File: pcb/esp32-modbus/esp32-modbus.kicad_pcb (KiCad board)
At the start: 2 copper layers, 77.5 x 77.9 mm, 54 parts, among them J1 Conn_01x01_Male, J10 Conn_01x01_Male, J12 Conn_01x01_Male, J13 Conn_01x01_Male, J2 Conn_01x05_Male, J22 Conn_01x01_Male, J23 Conn_01x01_Male, J24 Conn_01x01_Male, J25 Conn_01x01_Male, J26 Conn_01x01_Male, J27_VCC1 Conn_01x01_Male, J28_RO1 Conn_01x01_Male, J29_DI1 Conn_01x01_Male, J3 Conn_01x01_Male, J30_RE/DE1 Conn_01x01_Male, J31_GND1 Conn_01x01_Male, J4 Conn_01x01_Male, J5 Conn_01x01_Male, J6 Screw_Terminal_01x02, J7 Conn_01x09_Male, J8 Conn_01x09_Male, J9 Conn_01x01_Male, Q1 BC817, Q2 BC817, U1 ESP32-WROOM-32U

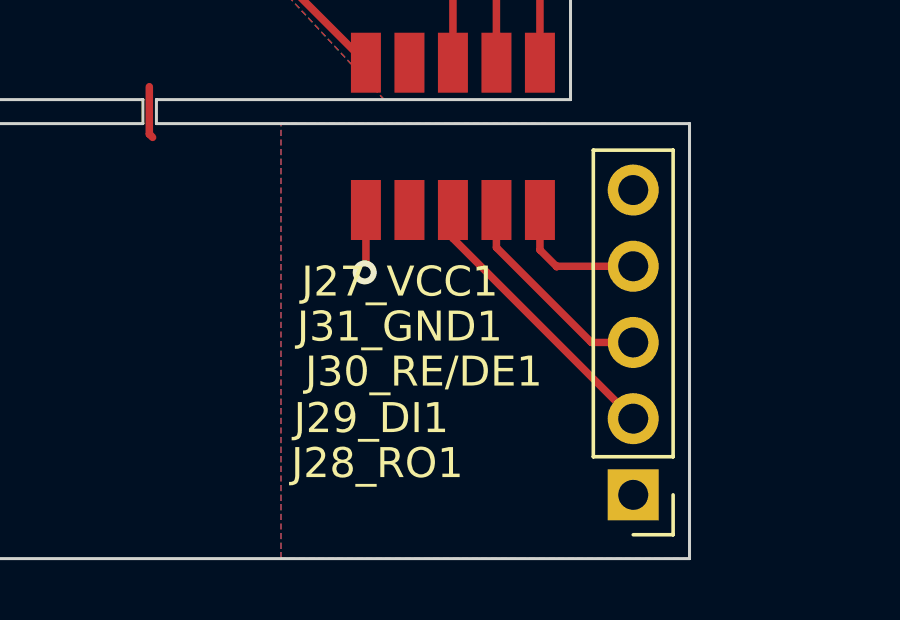
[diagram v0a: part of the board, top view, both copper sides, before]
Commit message: update
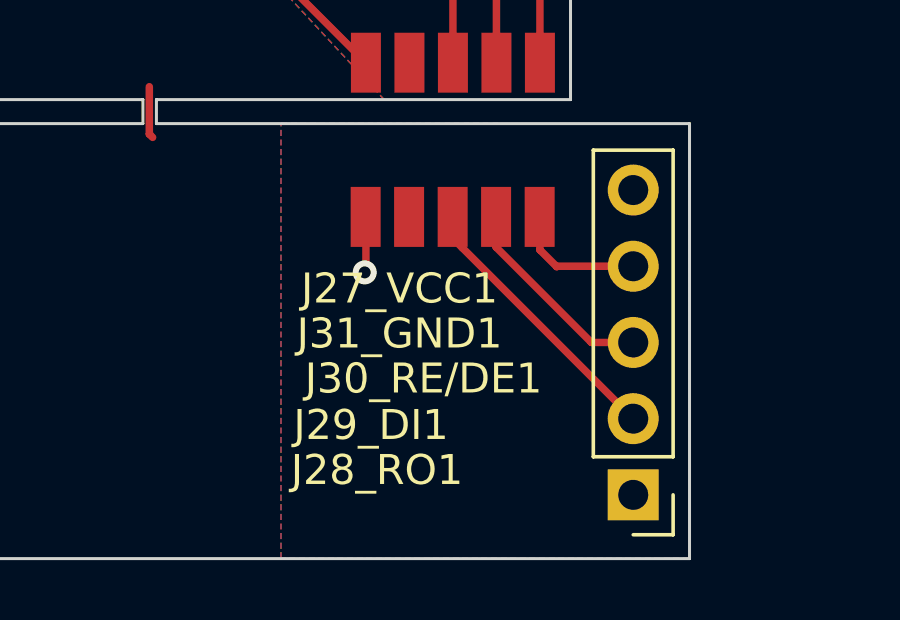
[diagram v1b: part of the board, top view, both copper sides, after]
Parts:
- moved J29_DI1 0.23 mm to (183.2, 136.3)
- moved J27_VCC1 0.23 mm to (178.9, 136.3)
- moved J28_RO1 0.23 mm to (184.7, 136.3)
- moved J30_RE/DE1 0.23 mm to (181.8, 136.3)
- moved J31_GND1 0.23 mm to (180.3, 136.3)
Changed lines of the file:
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@@
   )
   (footprint "custom:TestPoint_Pad_4.0x4.0mm2" (layer "F.Cu")
-    (at 183.24 136.03)
+    (at 183.23 136.26)
     (descr "SMD rectangular pad as test Point, square 4.0mm side length")
     (tags "test point SMD pad rectangle square")
@@
   )
   (footprint "custom:TestPoint_Pad_4.0x4.0mm2" (layer "F.Cu")
-    (at 178.89 136.03)
+    (at 178.88 136.26)
     (descr "SMD rectangular pad as test Point, square 4.0mm side length")
     (tags "test point SMD pad rectangle square")
@@
   )
   (footprint "custom:TestPoint_Pad_4.0x4.0mm2" (layer "F.Cu")
-    (at 184.69 136.03)
+    (at 184.68 136.26)
     (descr "SMD rectangular pad as test Point, square 4.0mm side length")
     (tags "test point SMD pad rectangle square")
@@
   )
   (footprint "custom:TestPoint_Pad_4.0x4.0mm2" (layer "F.Cu")
-    (at 181.79 136.03)
+    (at 181.78 136.26)
     (descr "SMD rectangular pad as test Point, square 4.0mm side length")
     (tags "test point SMD pad rectangle square")
@@
   )
   (footprint "custom:TestPoint_Pad_4.0x4.0mm2" (layer "F.Cu")
-    (at 180.34 136.03)
+    (at 180.33 136.26)
     (descr "SMD rectangular pad as test Point, square 4.0mm side length")
     (tags "test point SMD pad rectangle square")
@@
   (segment (start 172.26 74.11901) (end 173.435 72.94401) (width 0.25) (layer "B.Cu") (net 38))
   (segment (start 173.435 72.94401) (end 177.71401 72.94401) (width 0.25) (layer "B.Cu") (net 38))
-  (segment (start 181.74 135.98) (end 181.74 136.925) (width 0.25) (layer "F.Cu") (net 40))
-  (segment (start 181.74 136.925) (end 187.75 142.935) (width 0.25) (layer "F.Cu") (net 40))
-  (segment (start 186.355 140.395) (end 187.75 140.395) (width 0.25) (layer "F.Cu") (net 41))
-  (segment (start 183.19 137.23) (end 186.355 140.395) (width 0.25) (layer "F.Cu") (net 41))
-  (segment (start 183.19 135.98) (end 183.19 137.23) (width 0.25) (layer "F.Cu") (net 41))
-  (segment (start 184.64 135.98) (end 184.64 137.31) (width 0.25) (layer "F.Cu") (net 42))
+  (segment (start 182.0525 137.2375) (end 187.75 142.935) (width 0.25) (layer "F.Cu") (net 40))
+  (segment (start 181.73 136.915) (end 182.0525 137.2375) (width 0.25) (layer "F.Cu") (net 40))
+  (segment (start 181.73 136.21) (end 181.73 136.915) (width 0.25) (layer "F.Cu") (net 40))
+  (segment (start 182.0525 136.5325) (end 181.73 136.21) (width 0.25) (layer "F.Cu") (net 40))
+  (segment (start 183.18 137.22) (end 183.18 136.21) (width 0.25) (layer "F.Cu") (net 41))
+  (segment (start 187.75 140.395) (end 186.355 140.395) (width 0.25) (layer "F.Cu") (net 41))
+  (segment (start 186.355 140.395) (end 183.18 137.22) (width 0.25) (layer "F.Cu") (net 41))
+  (segment (start 184.64 137.31) (end 184.64 136.22) (width 0.25) (layer "F.Cu") (net 42))
   (segment (start 185.2 137.87) (end 185.215 137.855) (width 0.25) (layer "F.Cu") (net 42))
   (segment (start 185.215 137.855) (end 187.75 137.855) (width 0.25) (layer "F.Cu") (net 42))
+  (segment (start 184.64 136.22) (end 184.63 136.21) (width 0.25) (layer "F.Cu") (net 42))
   (segment (start 184.64 137.31) (end 185.2 137.87) (width 0.25) (layer "F.Cu") (net 42))
   (segment (start 178.84 135.98) (end 178.84 138.02) (width 0.25) (layer "F.Cu") (net 43))
